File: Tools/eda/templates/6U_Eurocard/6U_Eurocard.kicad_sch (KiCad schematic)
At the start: 1 part, among them J1 DIN41612_03x32_C_Split

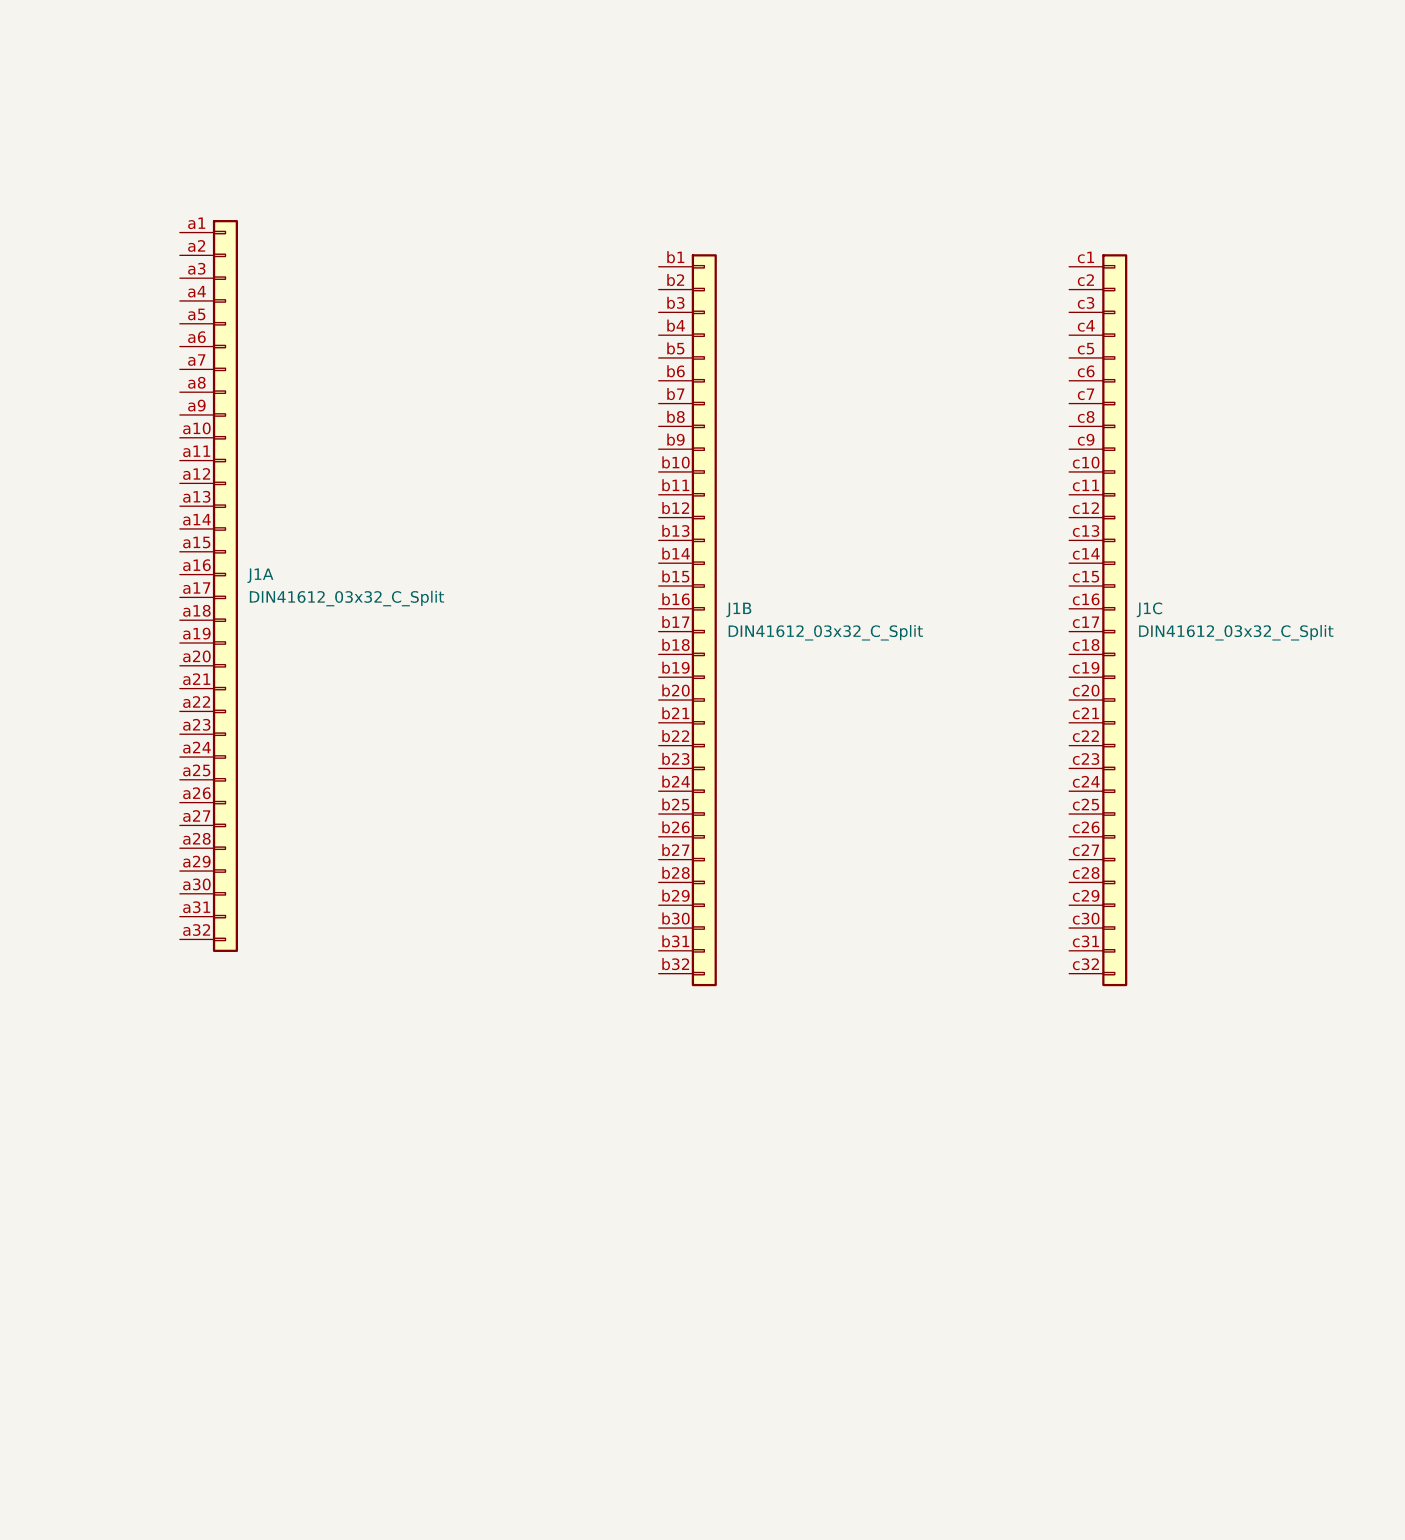
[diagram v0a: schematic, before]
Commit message: fixes
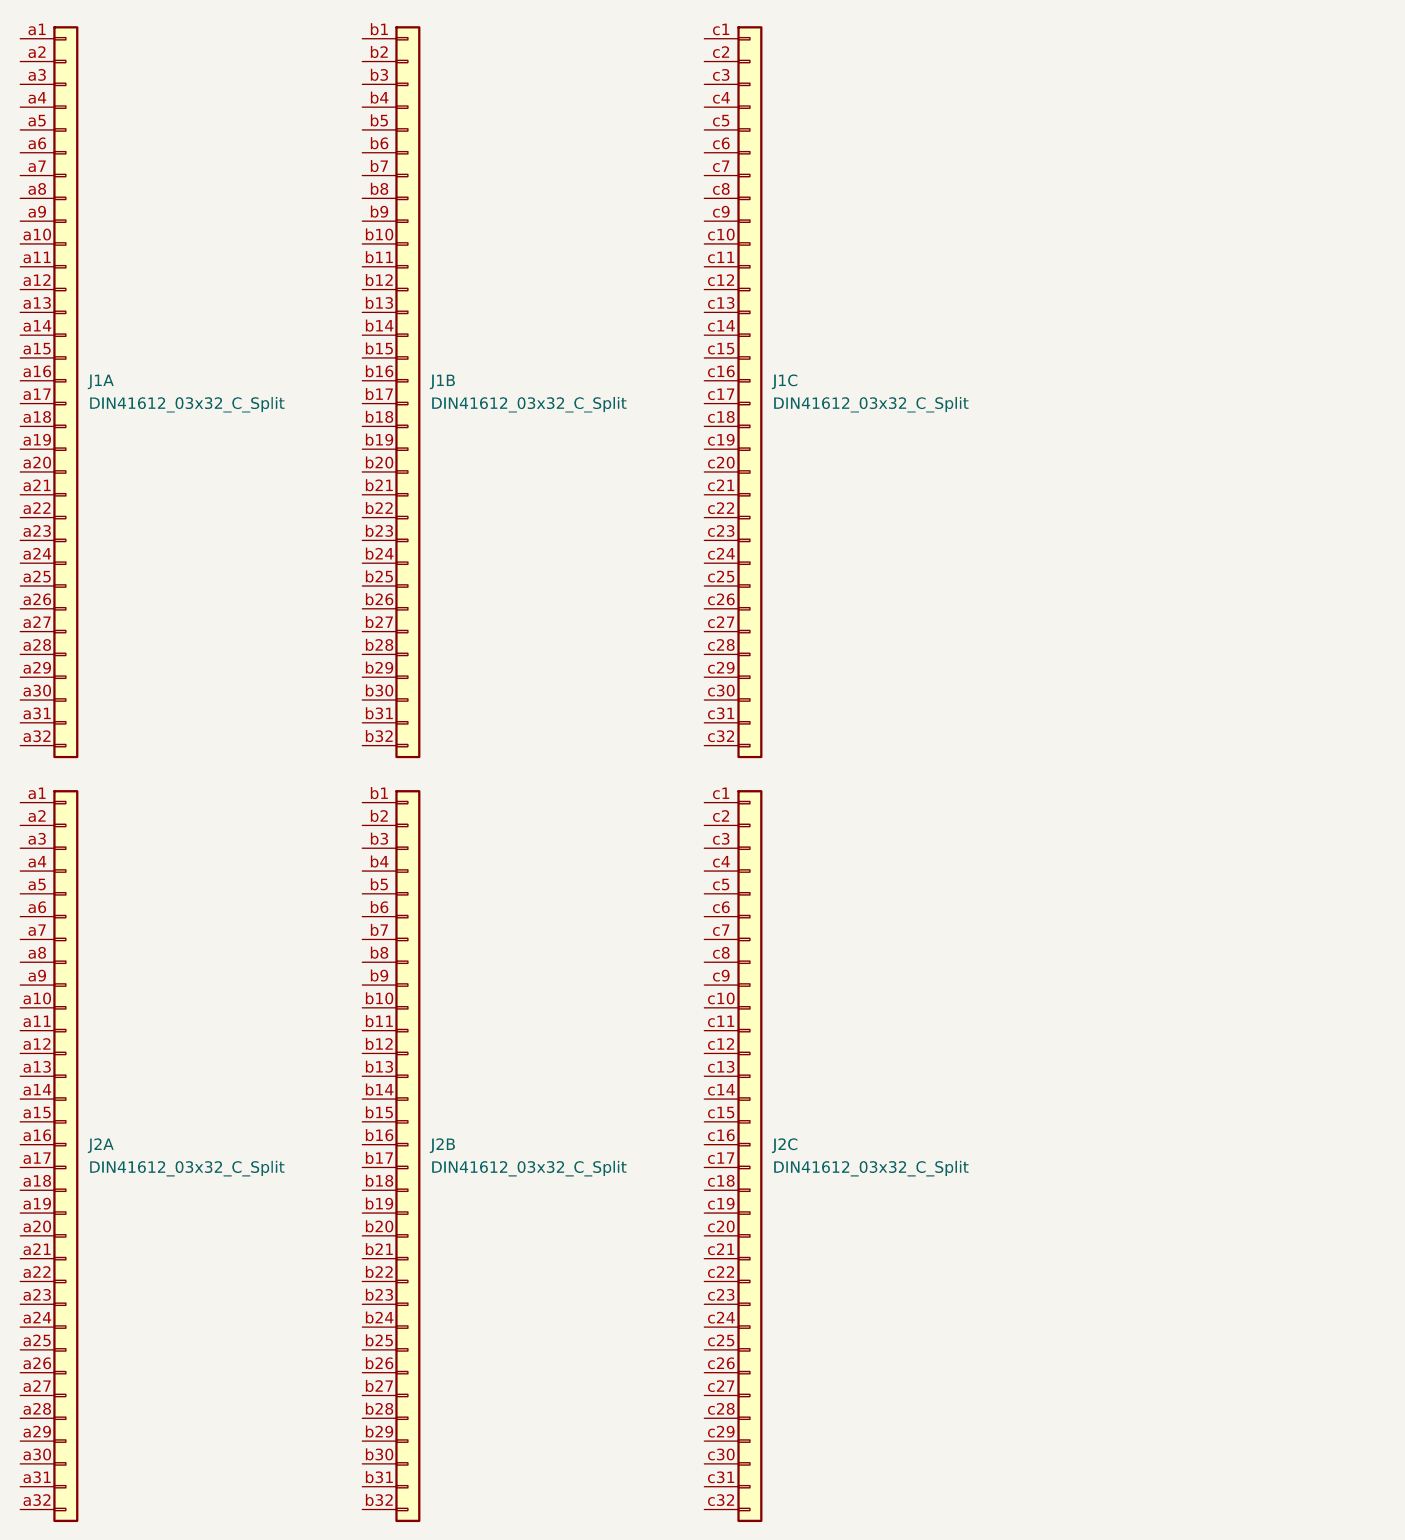
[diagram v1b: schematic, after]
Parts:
- added J2: DIN41612_03x32_C_Split, Connector_DIN:DIN41612_C_3x32_Male_Horizontal_THT, symbol Connector:DIN41612_03x32_C_Split
- J1: footprint Connector_DIN:DIN41612_C_3x32_Male_Horizontal_THT -> (none)
